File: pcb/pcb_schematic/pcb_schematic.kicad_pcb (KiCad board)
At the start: 4 copper layers, 30.2 x 47.8 mm, 33 parts, among them J1 Conn_ST_STDC14, J3 Conn_02x02_Odd_Even, J4 USB_B_Micro, Q1 MMBT3904, Q2 MMBT3904, Q3 MMBT3904, U1 STM32G031K8Tx, U2 NCP1117-3.3_SOT223, U4 SSD1306 128 x 64 OLED (0x3C), U5 TCS34725 (0x29), Y1 Crystal

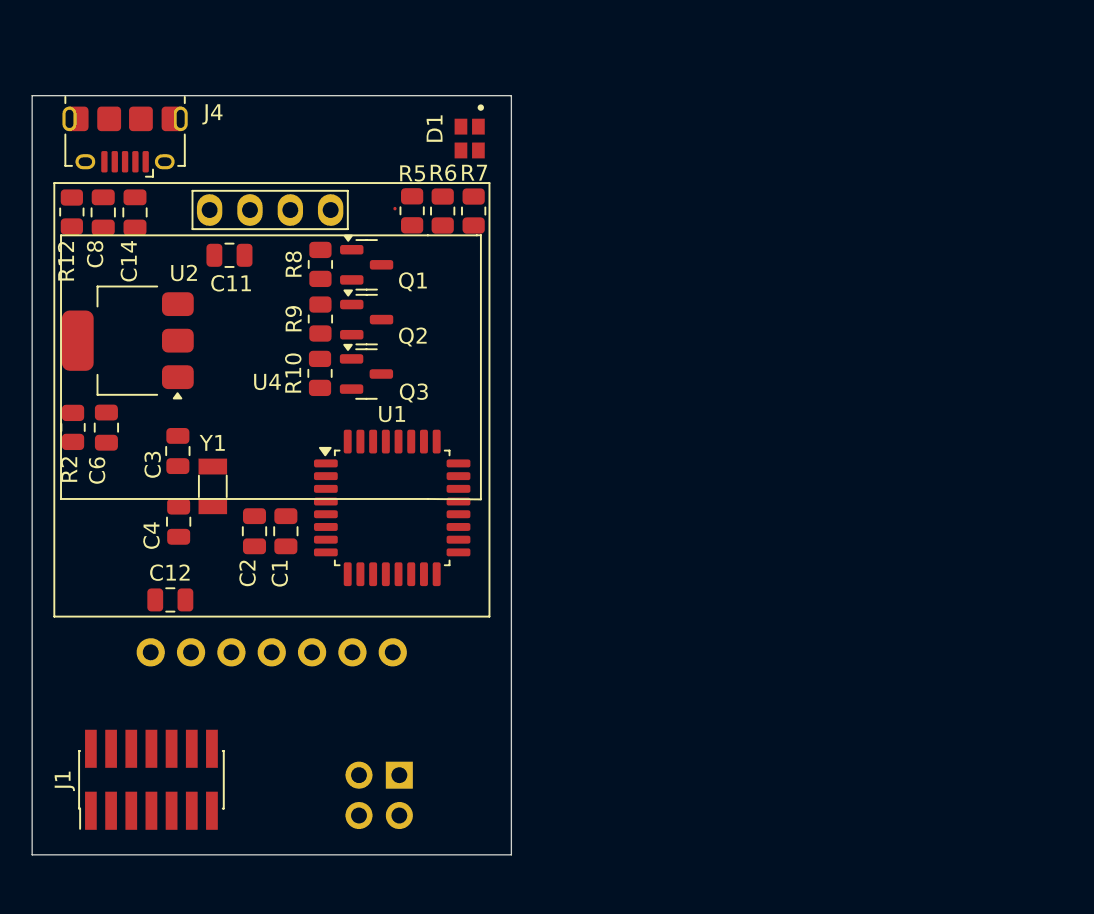
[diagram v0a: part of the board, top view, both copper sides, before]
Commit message: Update pcb_schematic.kicad_pcb
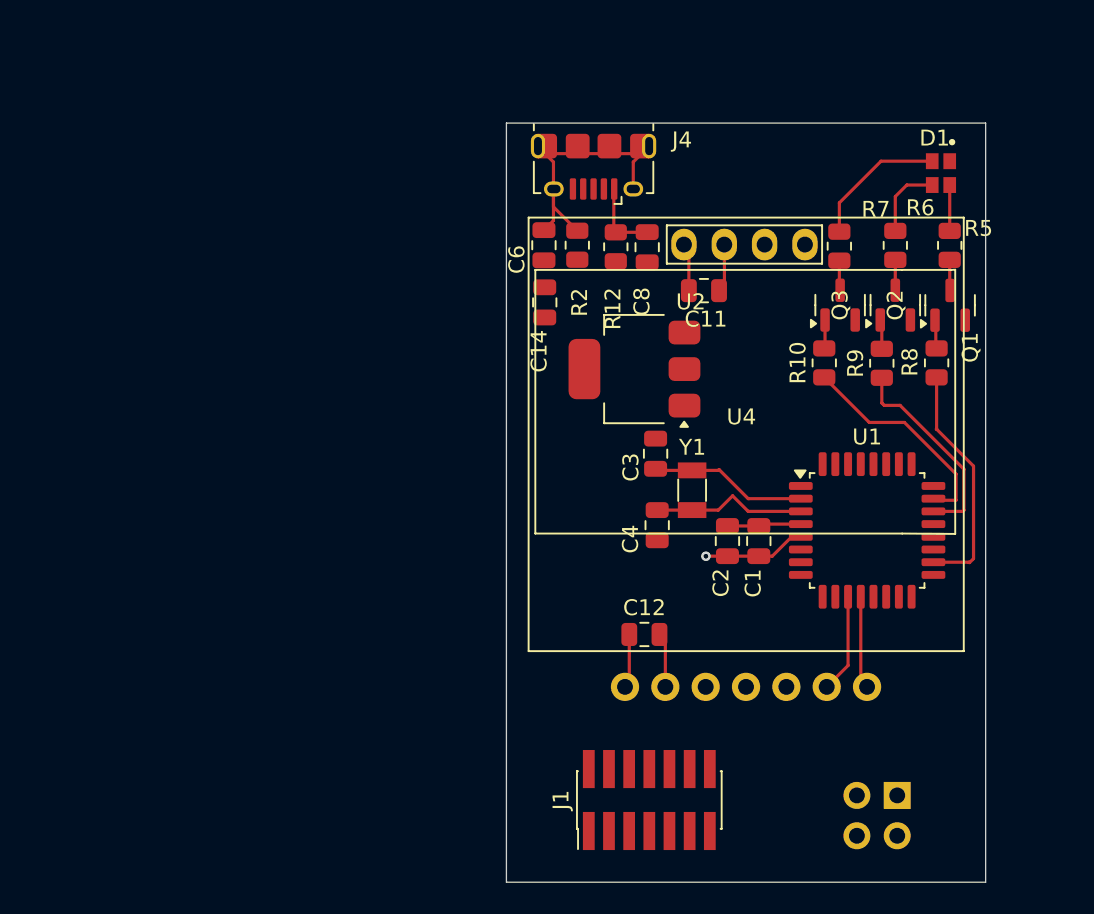
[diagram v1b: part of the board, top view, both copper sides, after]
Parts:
- moved R8 39.3 mm to (183.7, 86.6)
- moved Q1 36.8 mm to (184.6, 83.0), turned to 90 degrees
- moved R9 35.5 mm to (180.2, 86.6)
- moved R12 34.3 mm to (163.5, 79.3)
- moved C8 34.3 mm to (165.5, 79.3)
- moved R5 33.9 mm to (184.5, 79.2)
- moved R2 33.8 mm to (161.1, 79.2), turned to -90 degrees
- moved Q2 33.3 mm to (181.1, 83.0), turned to 90 degrees
- moved U2 32.0 mm to (164.7, 87.0)
- moved R10 31.8 mm to (176.6, 86.6)
- moved J1 31.4 mm to (165.6, 114.1)
- moved J3 31.4 mm to (181.2, 113.8)
- moved Y1 30.2 mm to (168.3, 94.6)
- moved Q3 30.1 mm to (177.6, 83.0), turned to 90 degrees
- moved C4 30.1 mm to (166.1, 96.8)
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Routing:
- net Net-(J4-Shield): track 0.00 -> 17.2 mm
- net PWM1: track 0.00 -> 15.0 mm
- net PWM3: track 0.00 -> 13.9 mm
- net PWM2: track 0.00 -> 13.0 mm
- net GND: track 0.00 -> 12.9 mm, vias 0 -> 1
- net +3.3V: track 0.00 -> 11.1 mm
- net Net-(U1-PC14): track 0.00 -> 9.97 mm
- net Net-(U1-PC15): track 0.00 -> 9.82 mm
- net Net-(D1-Pad4): track 0.00 -> 8.75 mm
- net INT: track 0.00 -> 6.23 mm
- net LED: track 0.00 -> 5.84 mm
- net Net-(D1-Pad3): track 0.03 -> 4.79 mm
- net VBUS: track 0.00 -> 4.28 mm
- net Net-(D1-Pad2): track 0.00 -> 2.89 mm
- net Net-(Q1-C): track 0.00 -> 1.94 mm
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- added copper zone on In1.Cu, net GND
